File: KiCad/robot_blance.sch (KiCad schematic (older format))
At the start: 6 parts, among them J1 Bat, U1 Esp32Dev, U2 MP1584, U3 MPU6050

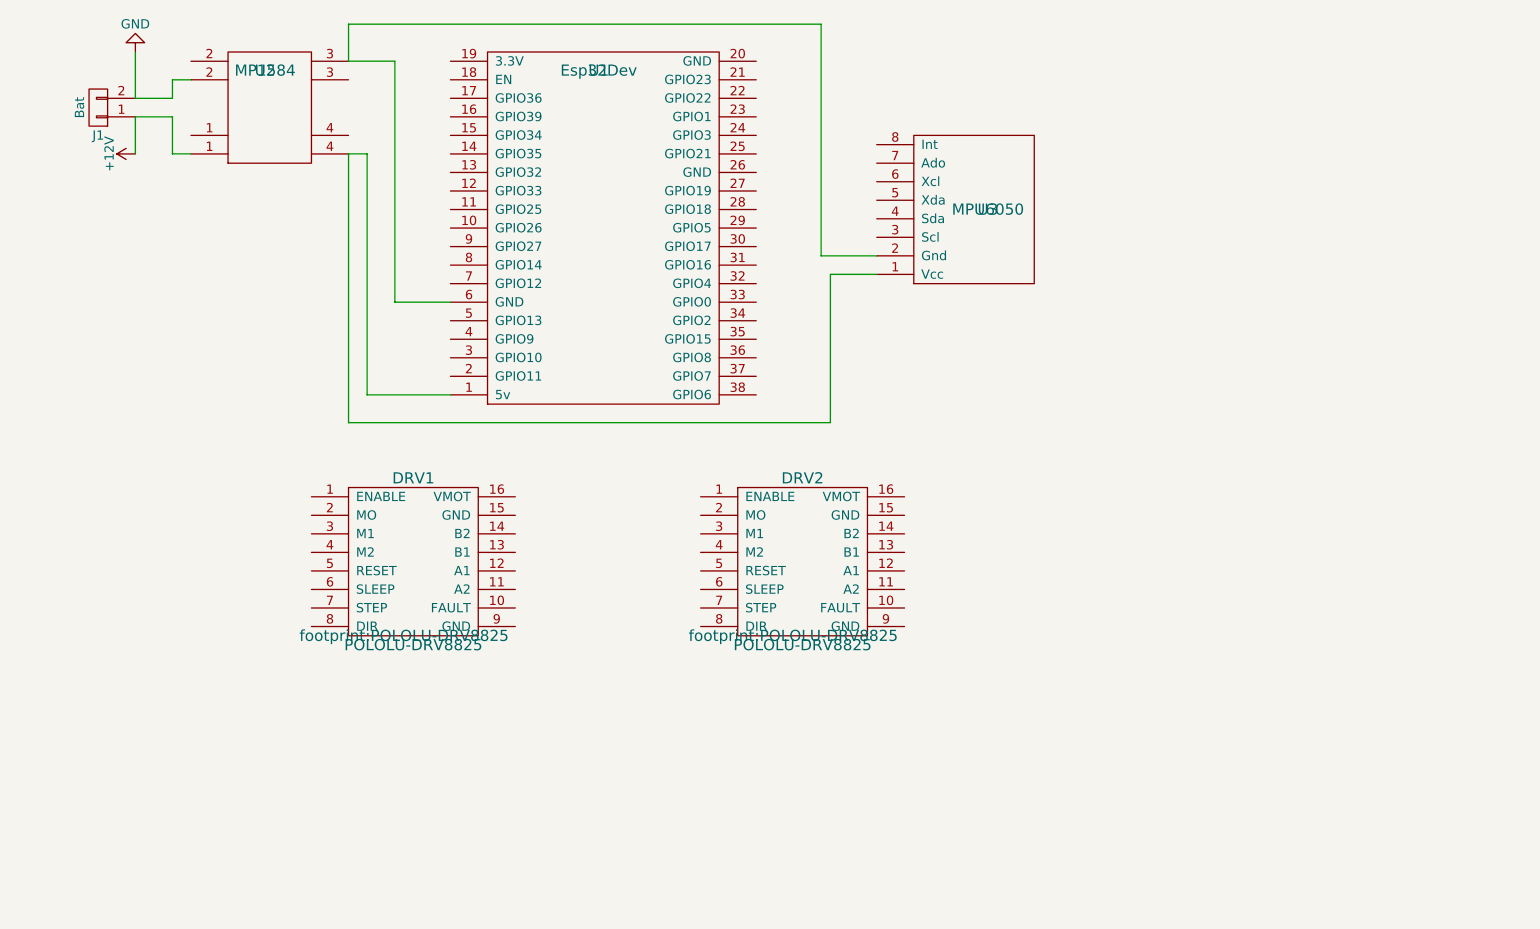
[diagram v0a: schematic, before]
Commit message: Servo
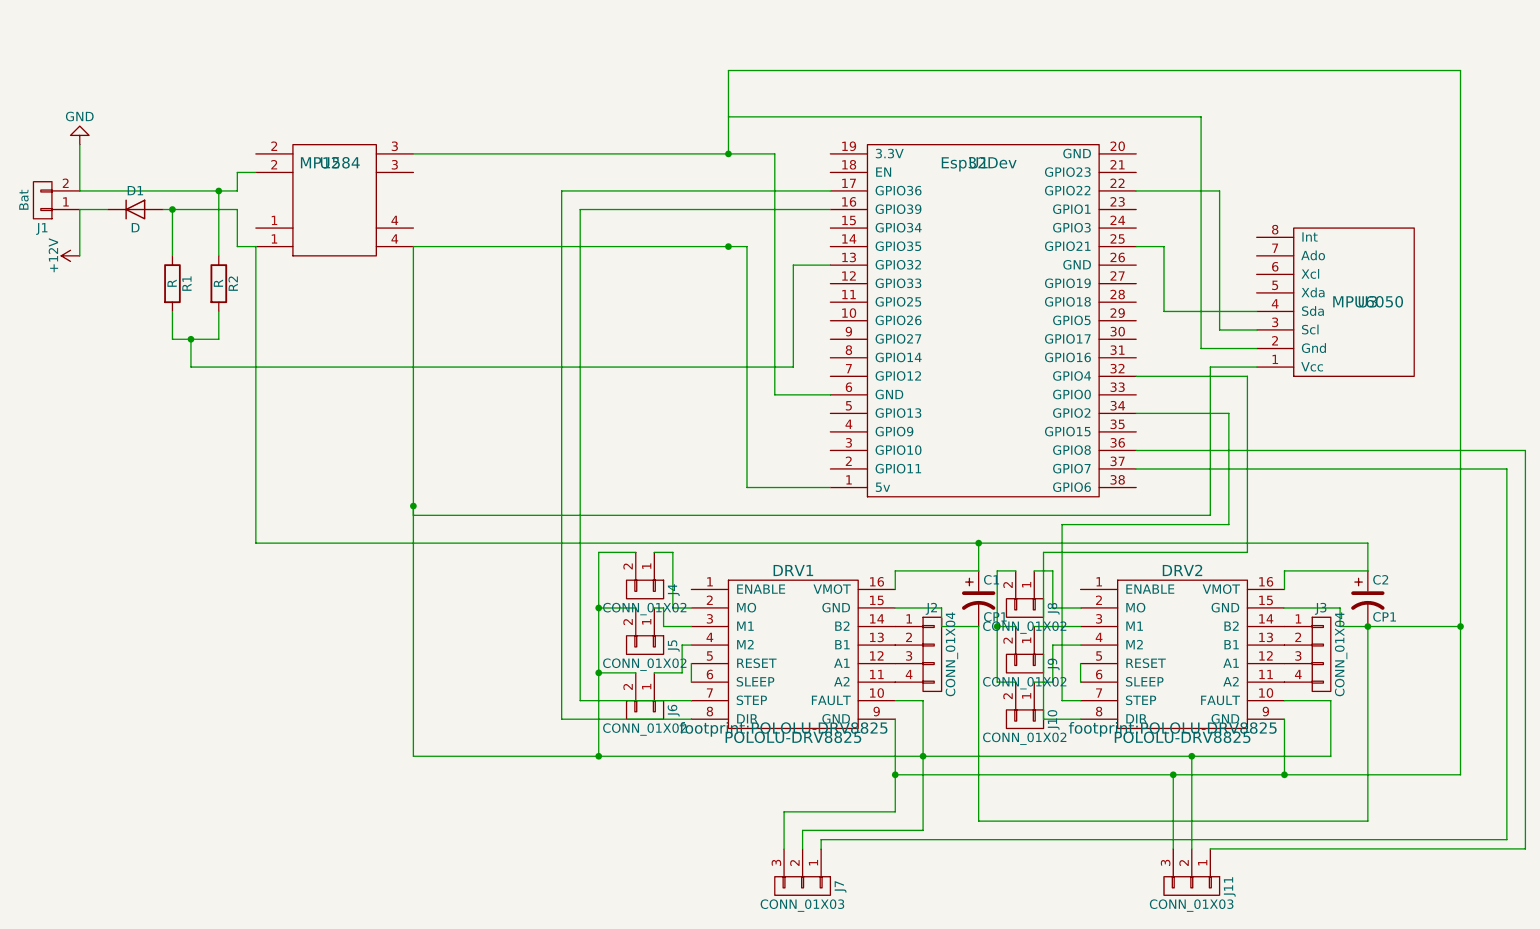
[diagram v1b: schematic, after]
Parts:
- added C1, C2: CP1, symbol CP1
- added D1: D, Diodes_THT:D_DO-41_SOD81_P7.62mm_Horizontal, symbol D
- added J10, J4, J5, J6, J8, J9: CONN_01X02, Connectors:PINHEAD1-2, symbol CONN_01X02
- added J11, J7: CONN_01X03, Connectors:PINHEAD1-3, symbol CONN_01X03
- added J2, J3: CONN_01X04, Connectors:Grove_1x04, symbol CONN_01X04
- added R1, R2: R, Resistors_THT:R_Axial_DIN0204_L3.6mm_D1.6mm_P5.08mm_Horizontal, symbol R
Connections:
- net +12V: now also D1.1 (K); no longer U2.1
- net GND: now also R2.1
- net at U1.1 (5v), U2.4, U3.1 (Vcc): now also DRV1.10 (FAULT), DRV2.10 (FAULT), J11.2 (P2), J4.2 (P2), J5.2 (P2), J6.2 (P2), J7.2 (P2)
- net at U1.13 (GPIO32): now also R1.2, R2.2
- net at U1.16 (GPIO39): now also DRV1.7 (STEP)
- net at U1.17 (GPIO36): now also DRV1.8 (DIR)
- net at U1.22 (GPIO22): now also U3.3 (Scl)
- net at U1.25 (GPIO21): now also U3.4 (Sda)
- net at U1.32 (GPIO4): now also DRV2.8 (DIR)
- net at U1.34 (GPIO2): now also DRV2.7 (STEP)
- net at U1.36 (GPIO8): now also J11.1 (P1)
- net at U1.37 (GPIO7): now also J7.1 (P1)
- net at DRV1.11 (A2): now also J2.4 (P4)
- net at DRV1.12 (A1): now also J2.3 (P3)
- net at DRV1.13 (B1): now also J2.2 (P2)
- net at DRV1.14 (B2): now also J2.1 (P1)
- net at DRV1.15 (GND): now also DRV1.9 (GND), DRV2.15 (GND), DRV2.9 (GND), U1.6 (GND), U2.3, C1.2, C2.2, J11.3 (P3), J7.3 (P3)
- net at DRV1.16 (VMOT): now also DRV2.16 (VMOT), U2.1, C1.1, C2.1, D1.2 (A), R1.1
- net at DRV1.2 (MO): now also J4.1 (P1)
- net at DRV1.3 (M1): now also J5.1 (P1)
- net at DRV1.4 (M2): now also J6.1 (P1)
- net at DRV1.5 (RESET): now also DRV1.6 (SLEEP)
- net at DRV2.11 (A2): now also J3.4 (P4)
- net at DRV2.12 (A1): now also J3.3 (P3)
- net at DRV2.13 (B1): now also J3.2 (P2)
- net at DRV2.14 (B2): now also J3.1 (P1)
- net at DRV2.2 (MO): now also J8.1 (P1)
- net at DRV2.3 (M1): now also J9.1 (P1)
- net at DRV2.4 (M2): now also J10.1 (P1)
- net at DRV2.5 (RESET): now also DRV2.6 (SLEEP)
- new net: J10.2 (P2), J8.2 (P2), J9.2 (P2)
- now unconnected: U2.3, U3.2 (Gnd)
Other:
- moved on the sheet: DRV1, DRV2, J1, U1, U2, U3
